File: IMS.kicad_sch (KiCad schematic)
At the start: 12 parts, among them Y3 ASE-xxxMHz

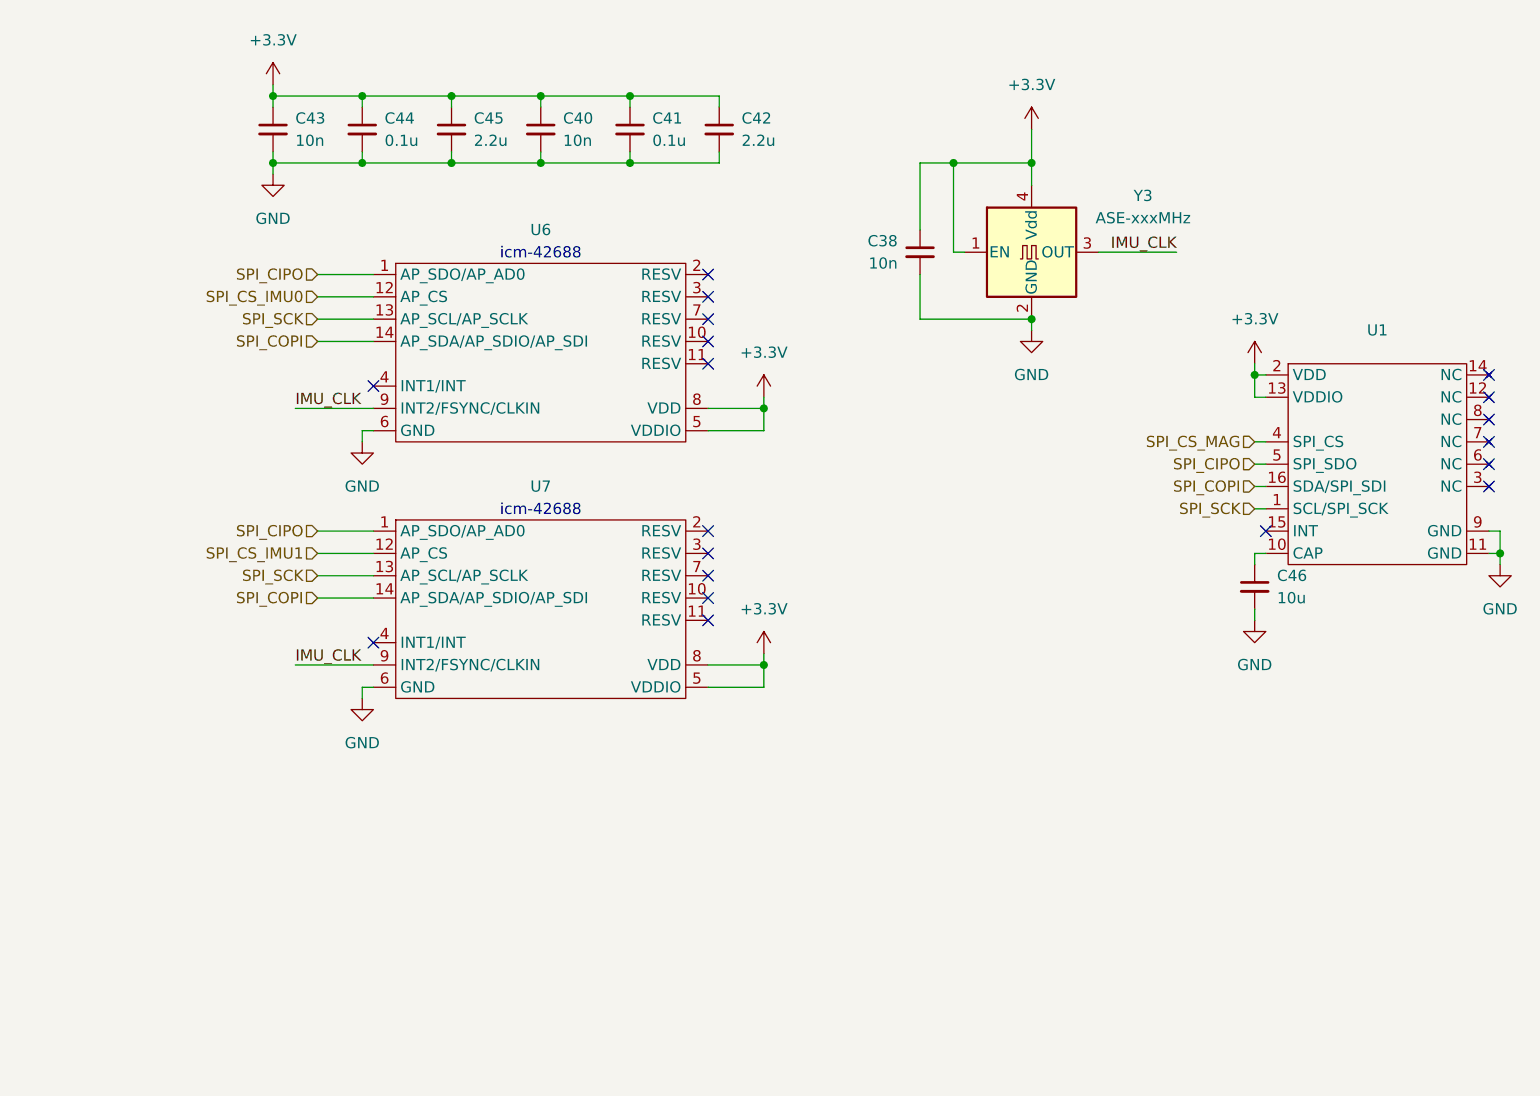
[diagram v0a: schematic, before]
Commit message: Finish IMS, finished more work on schematic
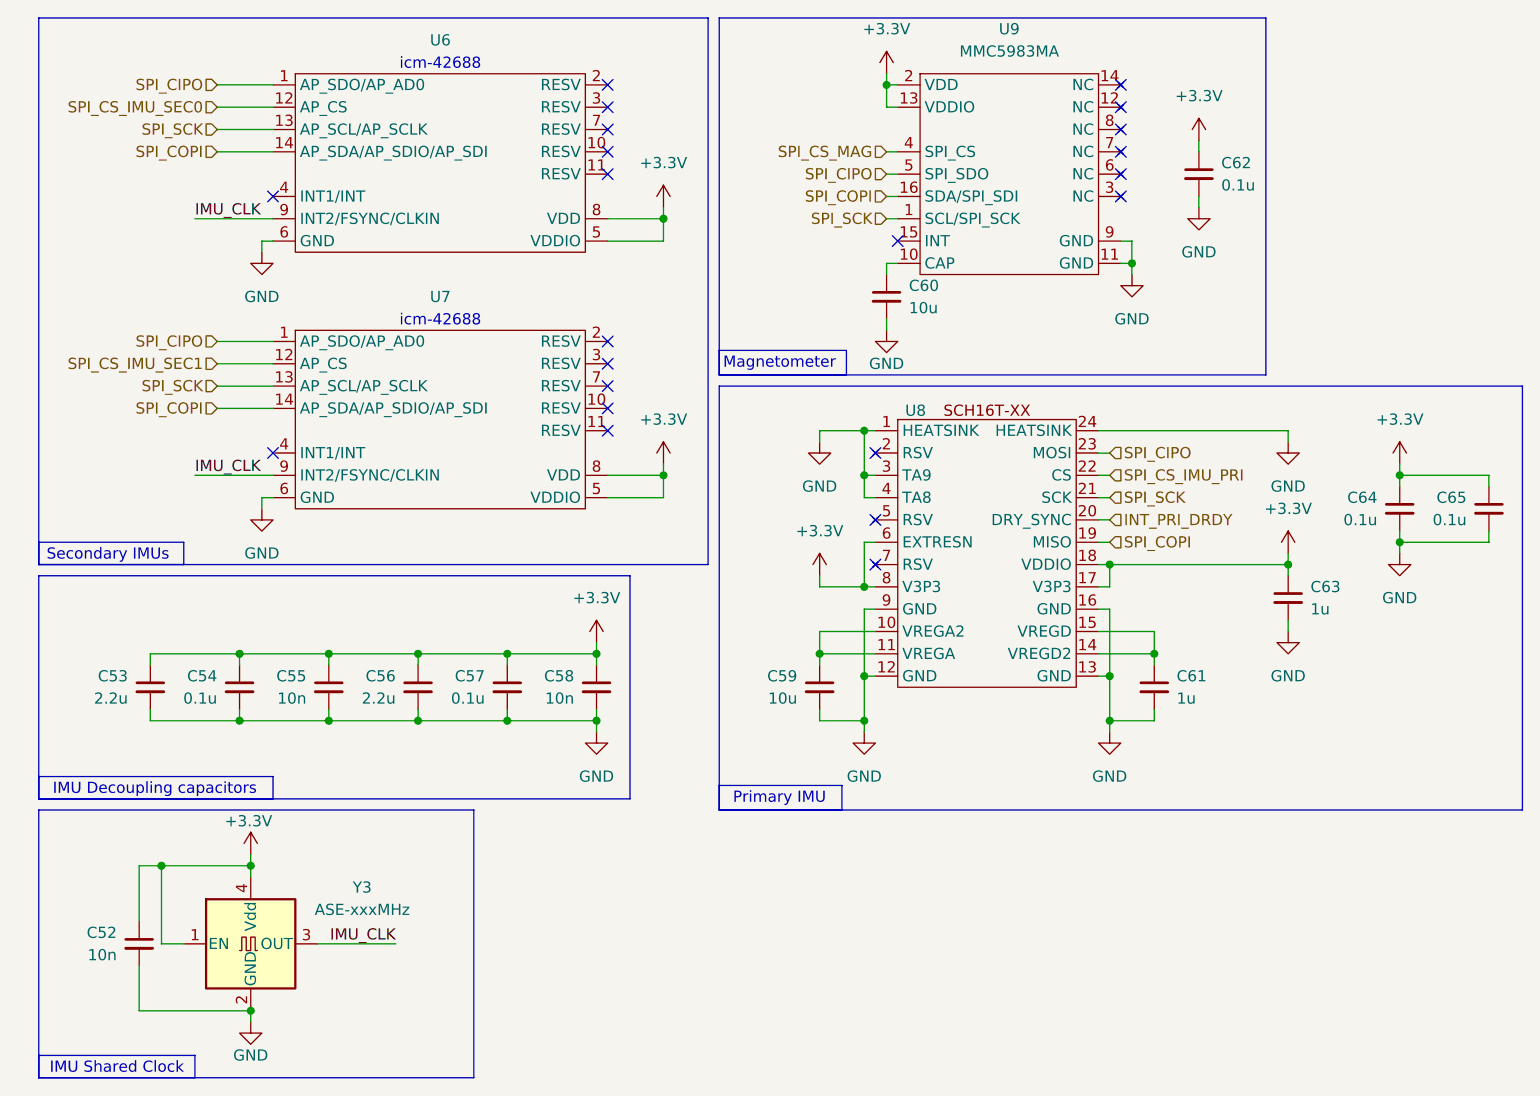
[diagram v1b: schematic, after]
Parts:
- added C59: 10u, Capacitor_SMD:C_0402_1005Metric, symbol Device:C_Small
- added C61, C63: 1u, Capacitor_SMD:C_0402_1005Metric, symbol Device:C_Small
- added C62, C64, C65: 0.1u, Capacitor_SMD:C_0402_1005Metric, symbol Device:C_Small
- added U8: ~, symbol SCH16T:SCH16T-XX
- C60: renamed from C46; footprint (none) -> Capacitor_SMD:C_0402_1005Metric
- U9: renamed from U1; value ~ -> MMC5983MA; footprint (none) -> Package_LGA:LGA-16_3x3mm_P0.5mm
- renumbered C38 to C52, C42 to C53, C41 to C54, C40 to C55, C45 to C56, C44 to C57, C43 to C58
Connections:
- net +3.3V: now also C62.1, C63.1, C64.1, C65.1, U8.17 (V3P3), U8.18 (VDDIO), U8.6 (EXTRESN), U8.8 (V3P3)
- net GND: now also C59.2, C61.2, C62.2, C63.2, C64.2, C65.2, U8.1 (HEATSINK), U8.12 (GND), U8.13 (GND), U8.16 (GND), U8.24 (HEATSINK), U8.3 (TA9), U8.4 (TA8), U8.9 (GND)
- net SPI_CIPO: now also U8.23 (MOSI)
- net SPI_COPI: now also U8.19 (MISO)
- net SPI_SCK: now also U8.21 (SCK)
- net SPI_CS_IMU0 renamed SPI_CS_IMU_SEC0
- net SPI_CS_IMU1 renamed SPI_CS_IMU_SEC1
- new net: C59.1, U8.10 (VREGA2), U8.11 (VREGA)
- new net: C61.1, U8.14 (VREGD2), U8.15 (VREGD)
- new net INT_PRI_DRDY: U8.20 (DRY_SYNC)
- new net SPI_CS_IMU_PRI: U8.22 (CS)
- no-connect marks 19 -> 22
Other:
- note added: "IMU Decoupling capacitors"
- note added: "IMU Shared Clock"
- note added: "Magnetometer"
- note added: "Primary IMU"
- note added: "Secondary IMUs"
- moved on the sheet: C52, C53, C54, C55, C56, C57, C58, C60, U6, U7, U9, Y3
